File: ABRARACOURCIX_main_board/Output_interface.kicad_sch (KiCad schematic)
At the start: 10 parts, among them J1 XT60PW-M, J10 Conn_01x03_Socket, J11 Conn_01x03_Socket, J8 Conn_01x03_Socket, J9 Conn_01x03_Socket, Q1 MMBT3904

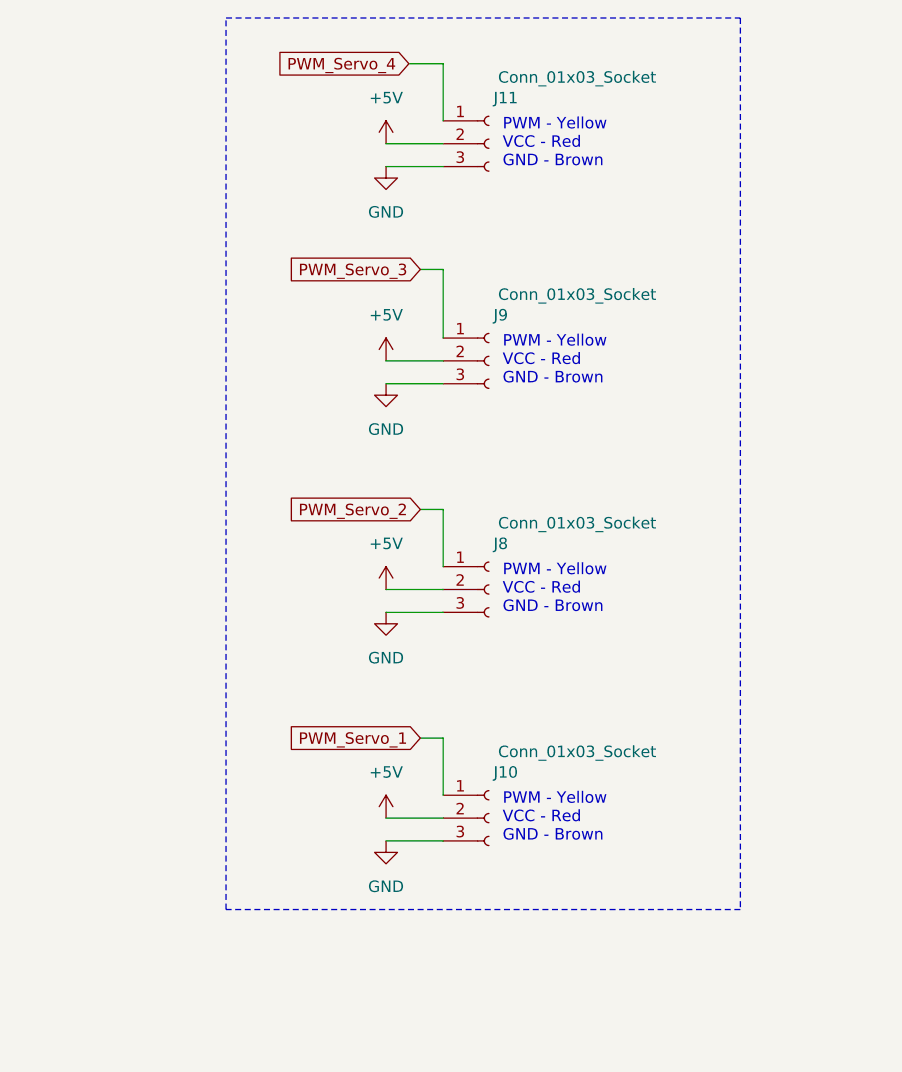
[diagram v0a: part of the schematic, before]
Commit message: Damn j'ai oublié de push y'a 2 semaines
je sais plus
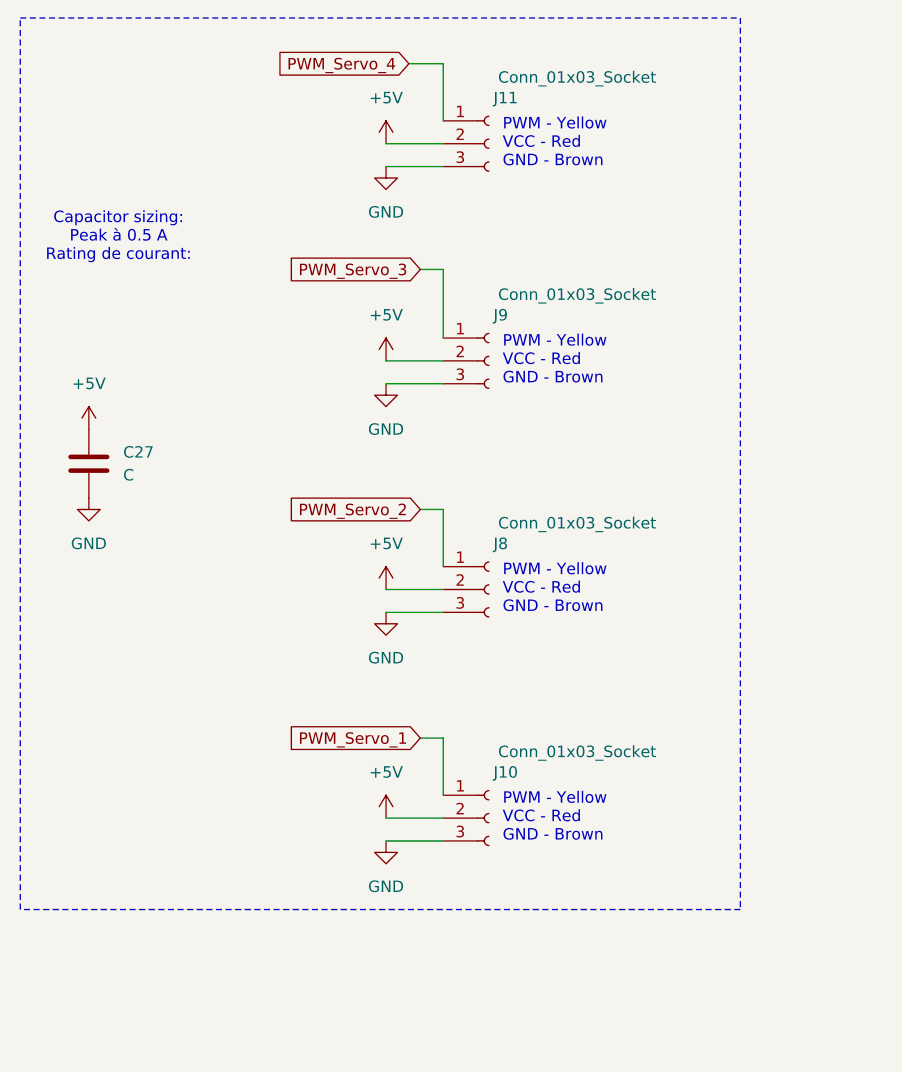
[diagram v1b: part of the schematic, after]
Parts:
- added C27: C, symbol Device:C
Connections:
- net +5V: now also C27.1
- net GND: now also C27.2
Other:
- note added: "Capacitor sizing: Peak à 0.5 A Rating de courant:"
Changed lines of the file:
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@@
 	)
 	(rectangle
-		(start 59.69 31.75)
+		(start 36.83 31.75)
 		(end 116.84 130.81)
 		(stroke
@@
 			)
 			(justify left)
+		)
+	)
+	(text "Capacitor sizing:\nPeak à 0.5 A\nRating de courant:"
+		(exclude_from_sim no)
+		(at 47.752 56.134 0)
+		(effects
+			(font
+				(size 1.27 1.27)
+			)
 		)
 	)
@@
 	)
 	(symbol
+		(lib_id "power:+5V")
+		(at 44.45 77.47 0)
+		(unit 1)
+		(exclude_from_sim no)
+		(in_bom yes)
+		(on_board yes)
+		(dnp no)
+		(fields_autoplaced yes)
+		(property "Reference" "#PWR045"
+			(at 44.45 81.28 0)
+			(effects
+				(font
+					(size 1.27 1.27)
+				)
+				(hide yes)
+			)
+		)
+		(property "Value" "+5V"
+			(at 44.45 72.39 0)
+			(effects
+				(font
+					(size 1.27 1.27)
+				)
+			)
+		)
+		(property "Footprint" ""
+			(at 44.45 77.47 0)
+			(effects
+				(font
+					(size 1.27 1.27)
+				)
+				(hide yes)
+			)
+		)
+		(property "Datasheet" ""
+			(at 44.45 77.47 0)
+			(effects
+				(font
+					(size 1.27 1.27)
+				)
+				(hide yes)
+			)
+		)
+		(property "Description" "Power symbol creates a global label with name \"+5V\""
+			(at 44.45 77.47 0)
+			(effects
+				(font
+					(size 1.27 1.27)
+				)
+				(hide yes)
+			)
+		)
+		(pin "1"
+		)
+		(instances
+			(project "ABRARACOURCIX_main_board"
+				(path "/0de7b960-2097-47c8-970c-7acab0ada146/f5120b67-a5cd-4c16-9638-751b3f9906f3"
+					(reference "#PWR045")
+					(unit 1)
+				)
+			)
+		)
+	)
+	(symbol
+		(lib_id "power:GND")
+		(at 44.45 85.09 0)
+		(unit 1)
+		(exclude_from_sim no)
+		(in_bom yes)
+		(on_board yes)
+		(dnp no)
+		(fields_autoplaced yes)
+		(property "Reference" "#PWR044"
+			(at 44.45 91.44 0)
+			(effects
+				(font
+					(size 1.27 1.27)
+				)
+				(hide yes)
+			)
+		)
+		(property "Value" "GND"
+			(at 44.45 90.17 0)
+			(effects
+				(font
+					(size 1.27 1.27)
+				)
+			)
+		)
+		(property "Footprint" ""
+			(at 44.45 85.09 0)
+			(effects
+				(font
+					(size 1.27 1.27)
+				)
+				(hide yes)
+			)
+		)
+		(property "Datasheet" ""
+			(at 44.45 85.09 0)
+			(effects
+				(font
+					(size 1.27 1.27)
+				)
+				(hide yes)
+			)
+		)
+		(property "Description" "Power symbol creates a global label with name \"GND\" , ground"
+			(at 44.45 85.09 0)
+			(effects
+				(font
+					(size 1.27 1.27)
+				)
+				(hide yes)
+			)
+		)
+		(pin "1"
+		)
+		(instances
+			(project "ABRARACOURCIX_main_board"
+				(path "/0de7b960-2097-47c8-970c-7acab0ada146/f5120b67-a5cd-4c16-9638-751b3f9906f3"
+					(reference "#PWR044")
+					(unit 1)
+				)
+			)
+		)
+	)
+	(symbol
 		(lib_id "Connector:Conn_01x03_Socket")
 		(at 88.9 95.25 0)
@@
 					(unit 1)
 				)
+			)
+		)
+	)
+	(symbol
+		(lib_id "Device:C")
+		(at 44.45 81.28 0)
+		(unit 1)
+		(exclude_from_sim no)
+		(in_bom yes)
+		(on_board yes)
+		(dnp no)
+		(fields_autoplaced yes)
+		(property "Reference" "C27"
+			(at 48.26 80.0099 0)
+			(effects
+				(font
+					(size 1.27 1.27)
+				)
+				(justify left)
+			)
+		)
+		(property "Value" "C"
+			(at 48.26 82.5499 0)
+			(effects
+				(font
+					(size 1.27 1.27)
+				)
+				(justify left)
+			)
+		)
+		(property "Footprint" ""
+			(at 45.4152 85.09 0)
+			(effects
+				(font
+					(size 1.27 1.27)
+				)
+				(hide yes)
+			)
+		)
+		(property "Datasheet" "~"
+			(at 44.45 81.28 0)
+			(effects
+				(font
+					(size 1.27 1.27)
+				)
+				(hide yes)
+			)
+		)
+		(property "Description" "Unpolarized capacitor"
+			(at 44.45 81.28 0)
+			(effects
+				(font
+					(size 1.27 1.27)
+				)
+				(hide yes)
+			)
+		)
+		(pin "2"
+		)
+		(pin "1"
+		)
+		(instances
+			(project ""
+				(path "/0de7b960-2097-47c8-970c-7acab0ada146/f5120b67-a5cd-4c16-9638-751b3f9906f3"
+					(reference "C27")
+					(unit 1)
+				)
